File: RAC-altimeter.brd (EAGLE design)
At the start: 160 x 100 mm, 30 parts, among them J3 CORTEX_DEBUG_SMD, U1 MAX32660GTP+, U2 BMI088, U3 BMP388, U4 W25N01GVZEIG_TR, Y1 32.768kHz

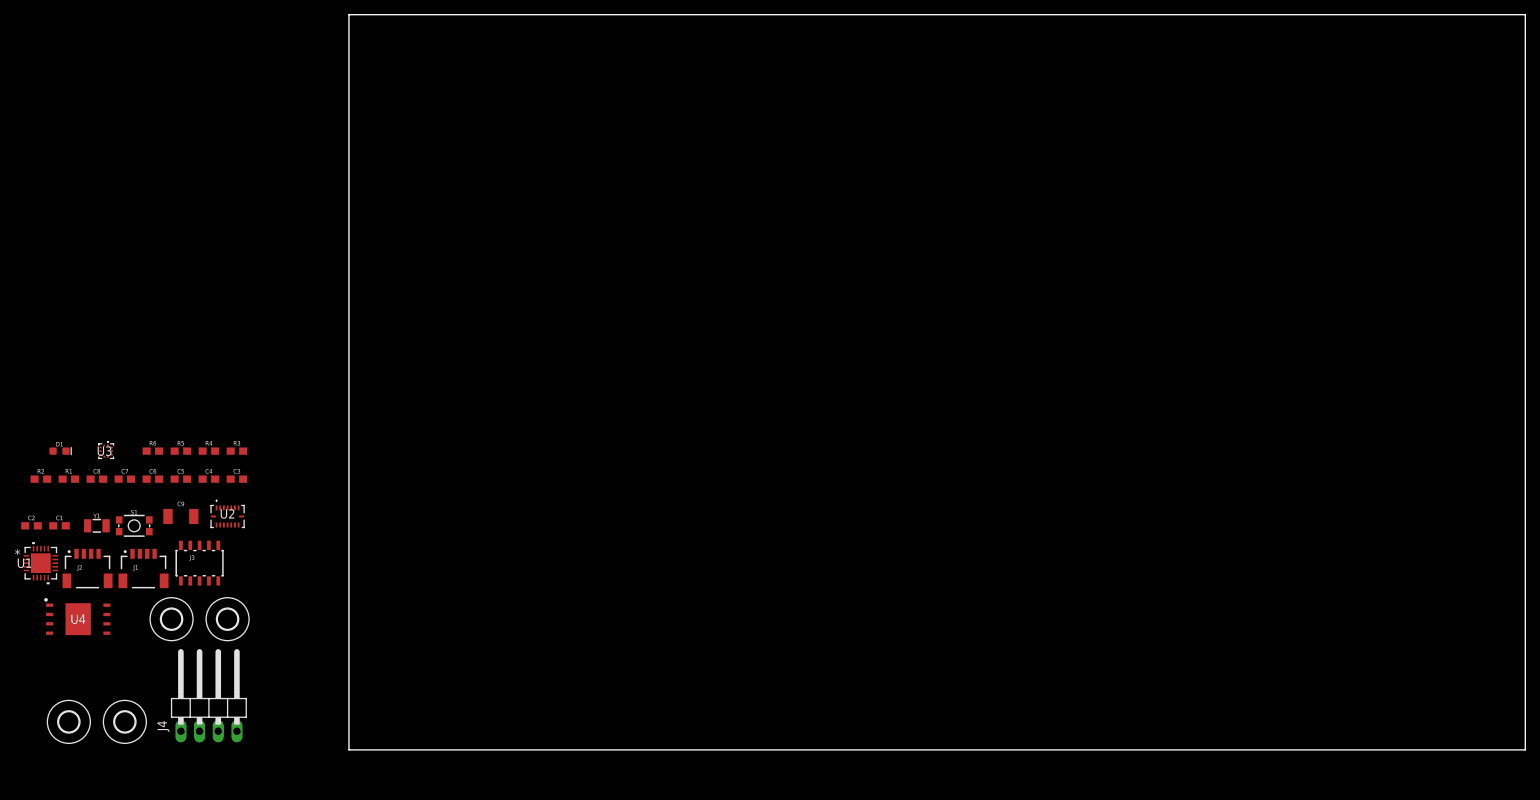
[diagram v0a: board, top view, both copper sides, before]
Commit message: Organized board for layout
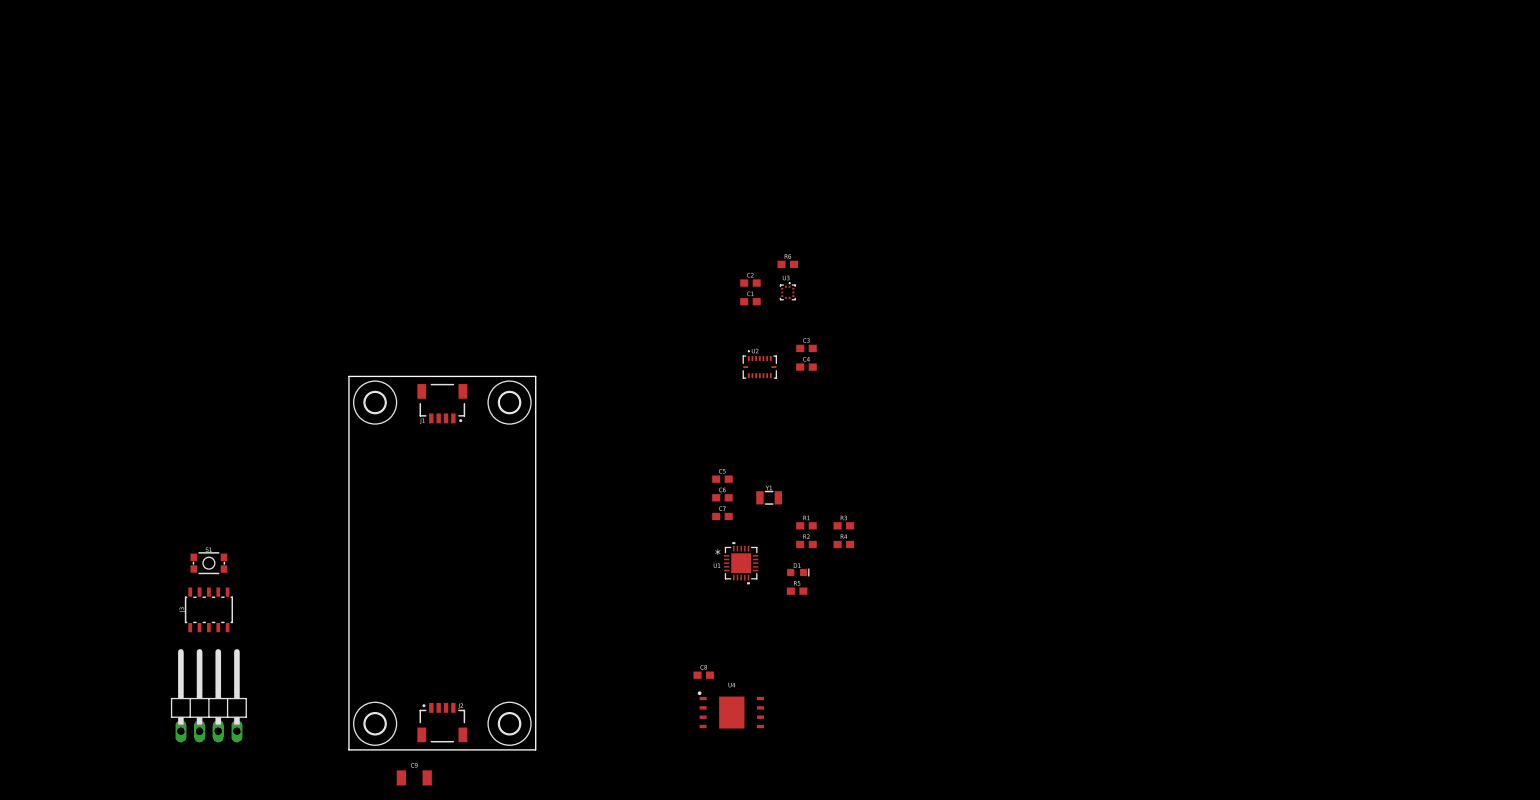
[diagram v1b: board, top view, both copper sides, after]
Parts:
- moved R2 104.5 mm to (62.2, 27.9)
- moved C2 103.2 mm to (54.6, 63.5)
- moved D1 101.7 mm to (61.0, 24.1)
- moved R1 100.5 mm to (62.2, 30.5)
- moved C1 98.8 mm to (54.6, 61.0)
- moved U1 95.2 mm to (53.3, 25.4)
- moved U3 95.2 mm to (59.7, 62.2)
- moved Y1 91.5 mm to (57.1, 34.3)
- moved R6 90.0 mm to (59.7, 66.0)
- moved U4 89.8 mm to (52.1, 5.08)
- moved R4 87.3 mm to (67.3, 27.9)
- moved C8 86.8 mm to (48.3, 10.2)
- moved R5 86.0 mm to (61.0, 21.6)
- moved R3 83.2 mm to (67.3, 30.5)
- moved C4 82.7 mm to (62.2, 52.1)
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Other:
- board size 160 x 100 mm -> 25.4 x 50.8 mm
